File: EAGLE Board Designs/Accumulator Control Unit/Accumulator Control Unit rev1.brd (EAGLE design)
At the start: 186.7 x 135.7 mm, 231 parts, among them J1 CONNECTOR-CAN_MF_T_V_, J2 CONNECTOR-8_MF_T_V_, J3 CONNECTOR-8_MF_T_V_, J4 CONNECTOR-2_MF_T_V_, J5 CONNECTOR-12_MF_T_V_, J6 CONNECTOR-14_MF_T_V_, Q1 TRANSISTOR_N_MOS__PMV15ENEA, Q2 TRANSISTOR_N_MOS__PMV15ENEA, Q3 TRANSISTOR_N_MOS__PMV15ENEA, Q4 TRANSISTOR_N_MOS__PMV15ENEA, T1 TRANSFORMER_HM2112ZNLT_AIRGAP, U1 RELAY_SOLIDSTATE_NO, U10 OPAMP_1_CHANNEL_OPA991, U11 LOGICGATE_AND_DCK3, U12 OPAMP_1_CHANNEL_OPA991, U13 OPAMP_1_CHANNEL_OPA991, U14 OPAMP_1_CHANNEL_OPA991, U15 LOGICGATE_AND_DCK3, U16 RELAY_SOLIDSTATE_NO, U17 VOLTAGE_REGULATOR_SOT223_3.3V, U18 OPAMP_1_CHANNEL_OPA991, U19 MAX7404, U2 ADG1423, U20 OPAMP_1_CHANNEL_OPA991, U22 OPAMP_1_CHANNEL_OPA991, U25 TCAN1051HQV-Q1, U26 MAX7404, U27 OPAMP_1_CHANNEL_OPA991, U28 MAX7404, U29 OPAMP_1_CHANNEL_OPA991, U3 LM555, U30 MAX7404, U4 OPAMP_1_CHANNEL_OPA991, U5 LTC6820, U6 ADM823, U7 OPAMP_1_CHANNEL_OPA991, U8 LOGICGATE_AND_DCK3, U9 OPAMP_1_CHANNEL_OPA991

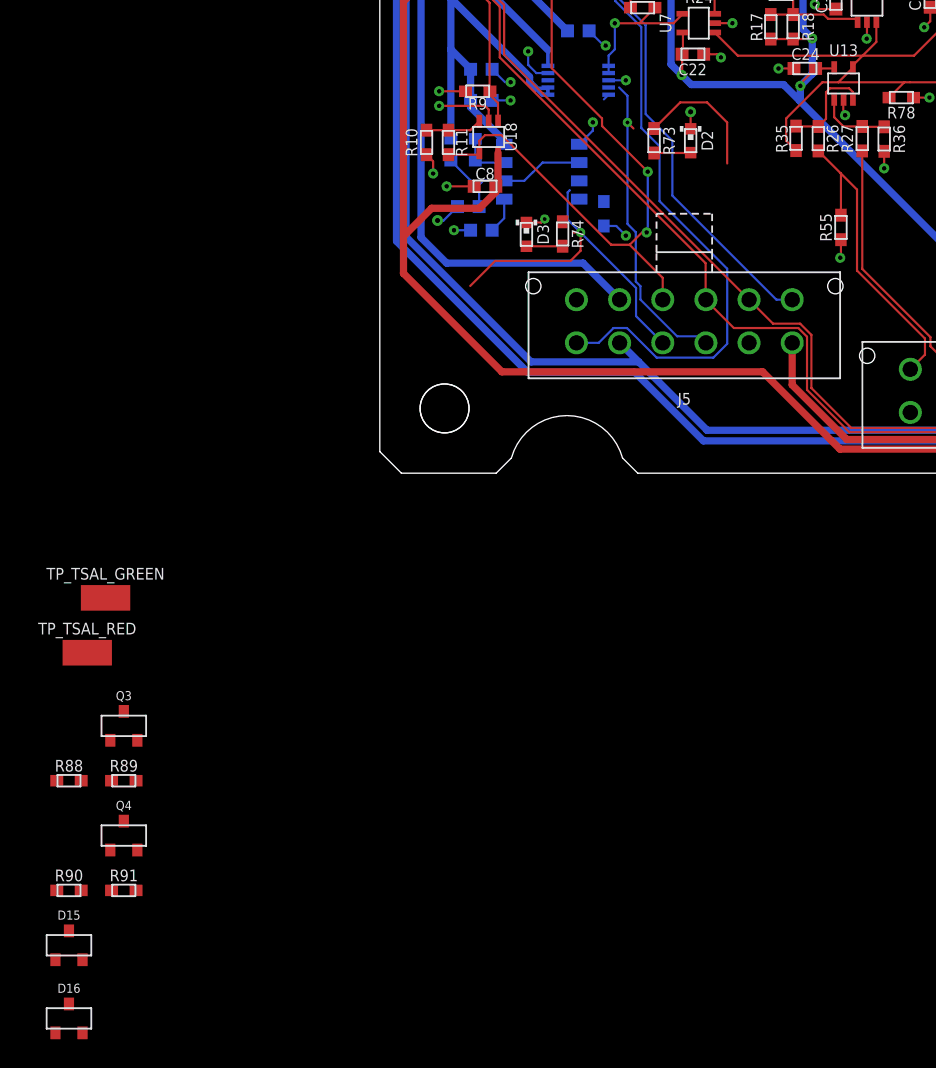
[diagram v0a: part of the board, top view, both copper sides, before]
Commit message: change names of revs
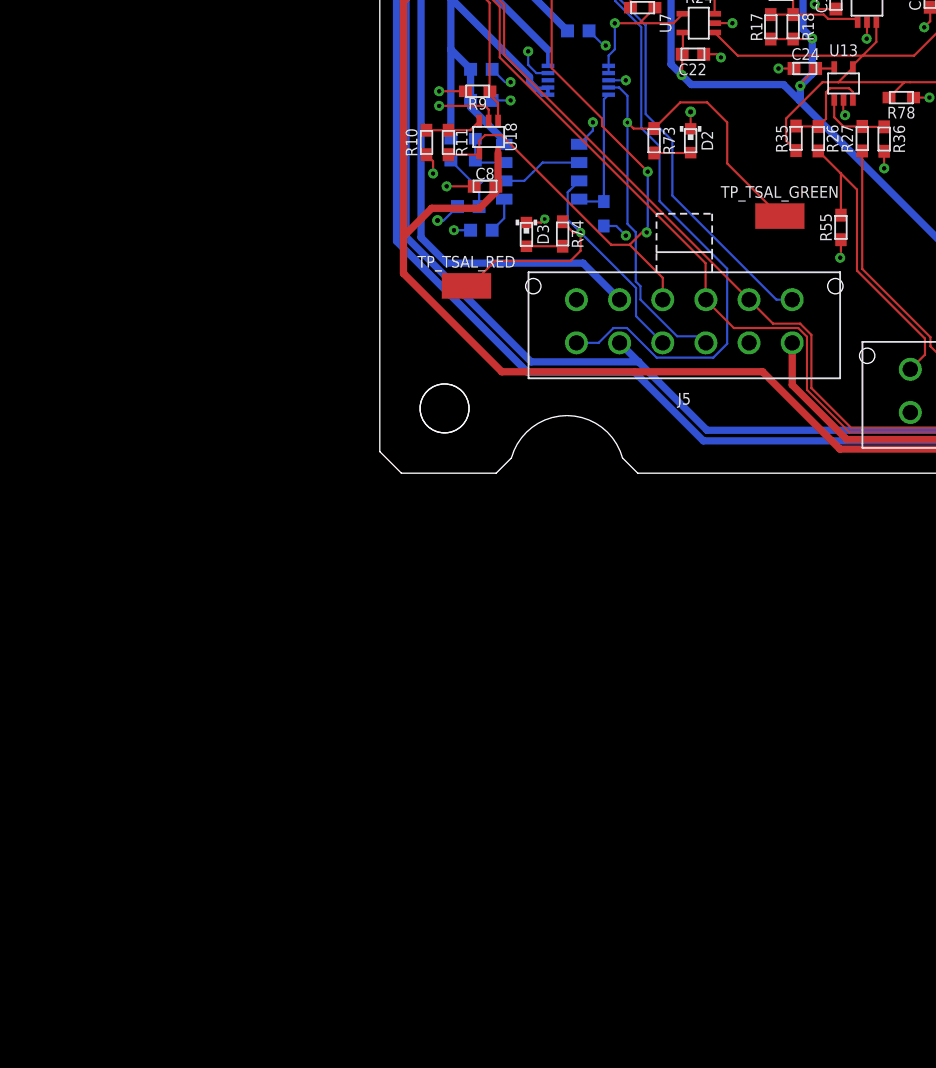
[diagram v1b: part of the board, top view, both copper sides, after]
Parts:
- removed D15, D16: TVS_15V, HyTechDevices:SOT-23
- removed Q3, Q4: TRANSISTOR_N_MOS__PMV15ENEA, HyTechDevices:SOT-23
- removed R88, R90: RESISTOR_0603_10, HyTechDevices:0603-RES
- removed R89, R91: RESISTOR_0603_10K, HyTechDevices:0603-RES
- moved TP_TSAL_GREEN 53.8 mm to (27.8, 16.4)
- moved TP_TSAL_RED 36.6 mm to (6.02, 11.5)
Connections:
- removed net N$60: Q3.1, R88.2
- removed net N$61: Q4.1, R90.2
- removed net TSAL_GREEN1: D15.3, R90.1, R91.1, TP_TSAL_GREEN.1, U2.9
- removed net TSAL_RED1: D16.3, R88.1, R89.1, TP_TSAL_RED.1, U3.3
- net +12V: no longer R73.1, R74.1
- net GND: now also D2.1, D3.1; no longer D15.1, D16.1, Q3.2, Q4.2, R89.2, R91.2
- net TSAL_GREEN: now also R73.1, TP_TSAL_GREEN.1, U2.9; no longer D2.1, Q4.3
- net TSAL_RED: now also R74.1, TP_TSAL_RED.1, U3.3; no longer D3.1, Q3.3
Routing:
- net TSAL_GREEN: track 22.9 -> 38.3 mm, vias 2 -> 1
- net +12V: track 592.7 -> 583.5 mm
- net TIMER_EN: track 0.70 -> 9.34 mm
- net GND: track 205.6 -> 208.2 mm, vias 155 -> 157
- net TSAL_RED: track 25.2 -> 26.1 mm, vias 2 -> 1
